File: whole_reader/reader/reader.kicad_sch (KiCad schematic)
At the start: 59 parts, among them J1 Speaker+, J2 Speaker-, J3 Conn_02x05_Odd_Even, J4 USB_C_Receptacle_USB2.0_14P, J5 RFID RC522, J6 6P6C, SW1 SW_SPDT, SW2 SW_SPDT, U1 LM386, U2 STM32F103C8T6, U3 MCP16301Hx-xCH, U4 MAX3232, Y1 16MHz

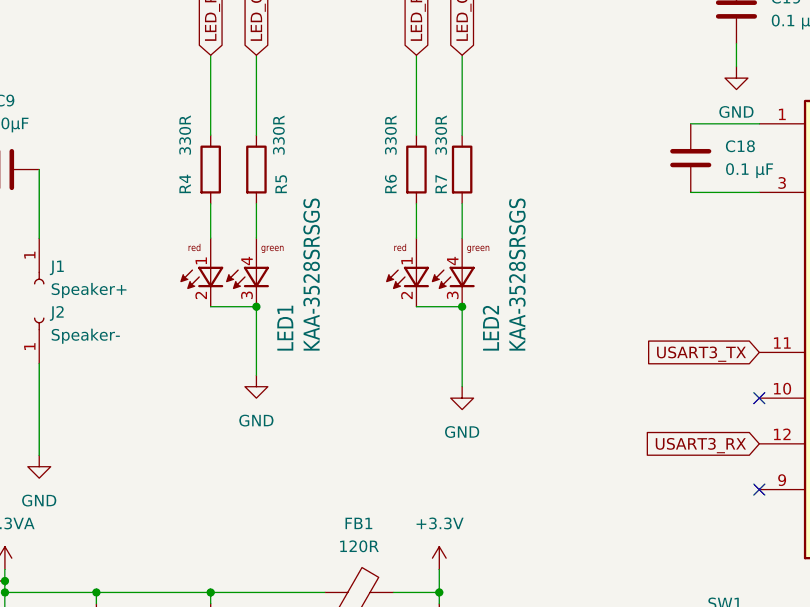
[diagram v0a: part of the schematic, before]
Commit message: minor changes in pcb layout
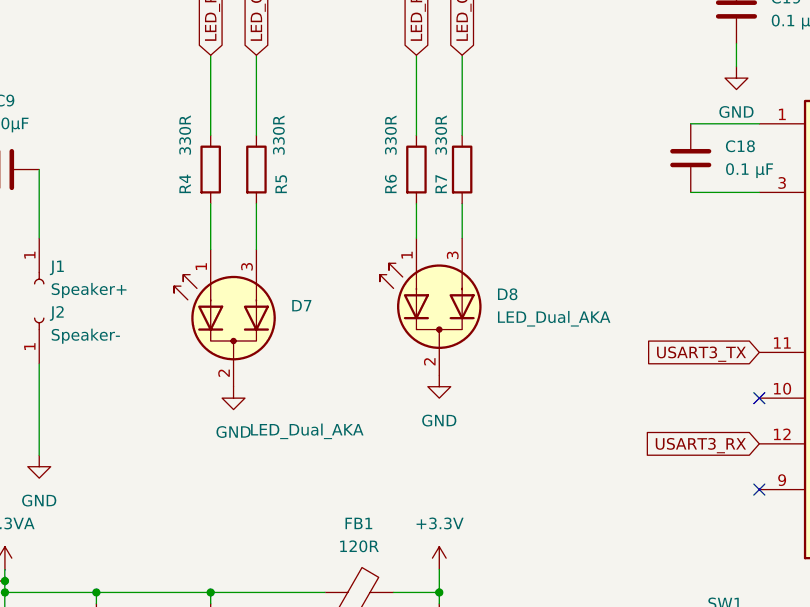
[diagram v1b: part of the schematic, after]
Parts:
- removed LED1, LED2: KAA-3528SRSGS, LED_SMD:LED_PLCC-2_3x2mm_KA, symbol deadlock-reader-eagle-import:KAA-3528SRSGS
- added D7, D8: LED_Dual_AKA, LED_SMD:LED_Kingbright_KPA-3010_3x2x1mm, symbol Device:LED_Dual_AKA
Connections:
- net GND: now also D7.2 (K), D8.2 (K)
- net at R4.2: now also D7.1 (A1)
- net at R5.2: now also D7.3 (A2)
- net at R6.2: now also D8.1 (A1)
- net at R7.2: now also D8.3 (A2)
